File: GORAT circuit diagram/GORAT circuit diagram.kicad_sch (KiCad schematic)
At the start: 78 parts, among them J1 AudioJack2, J2 AudioJack2, J3 Conn_01x08_Socket, J4 Conn_01x08_Socket, J6 Barrel_Jack, J8 Conn_01x02_Socket, J9 Conn_01x02_Socket, Q1 J111, SW1 SW_DPDT_x2, SW8 SW_Rotary2x6, U1 OP07CP, U2 TL072ACP, U3 TL072ACP

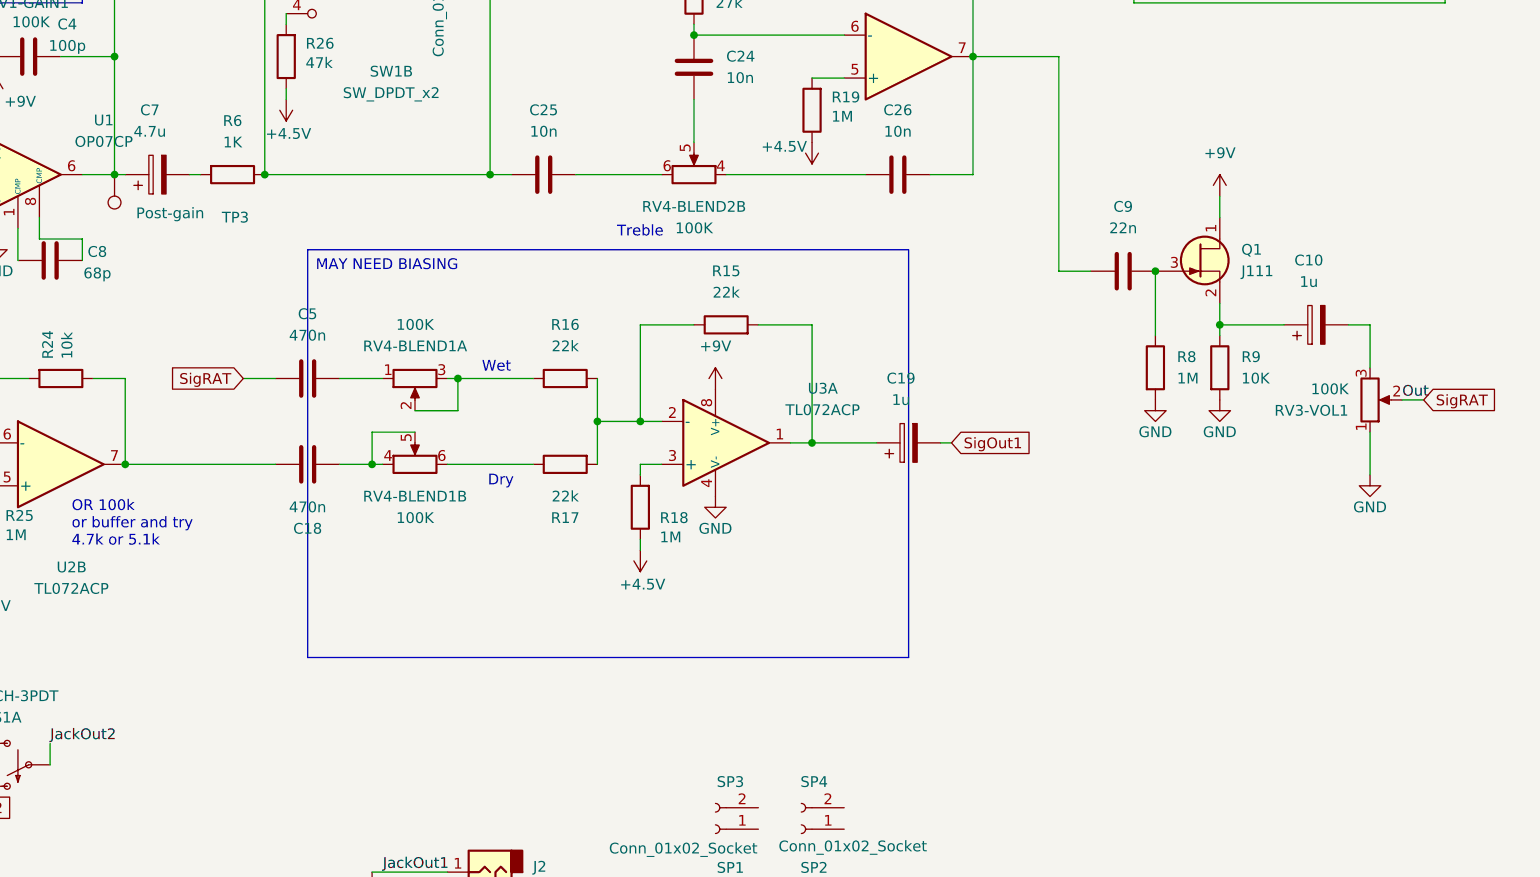
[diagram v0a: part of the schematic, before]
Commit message: potentially fixed volume mixer
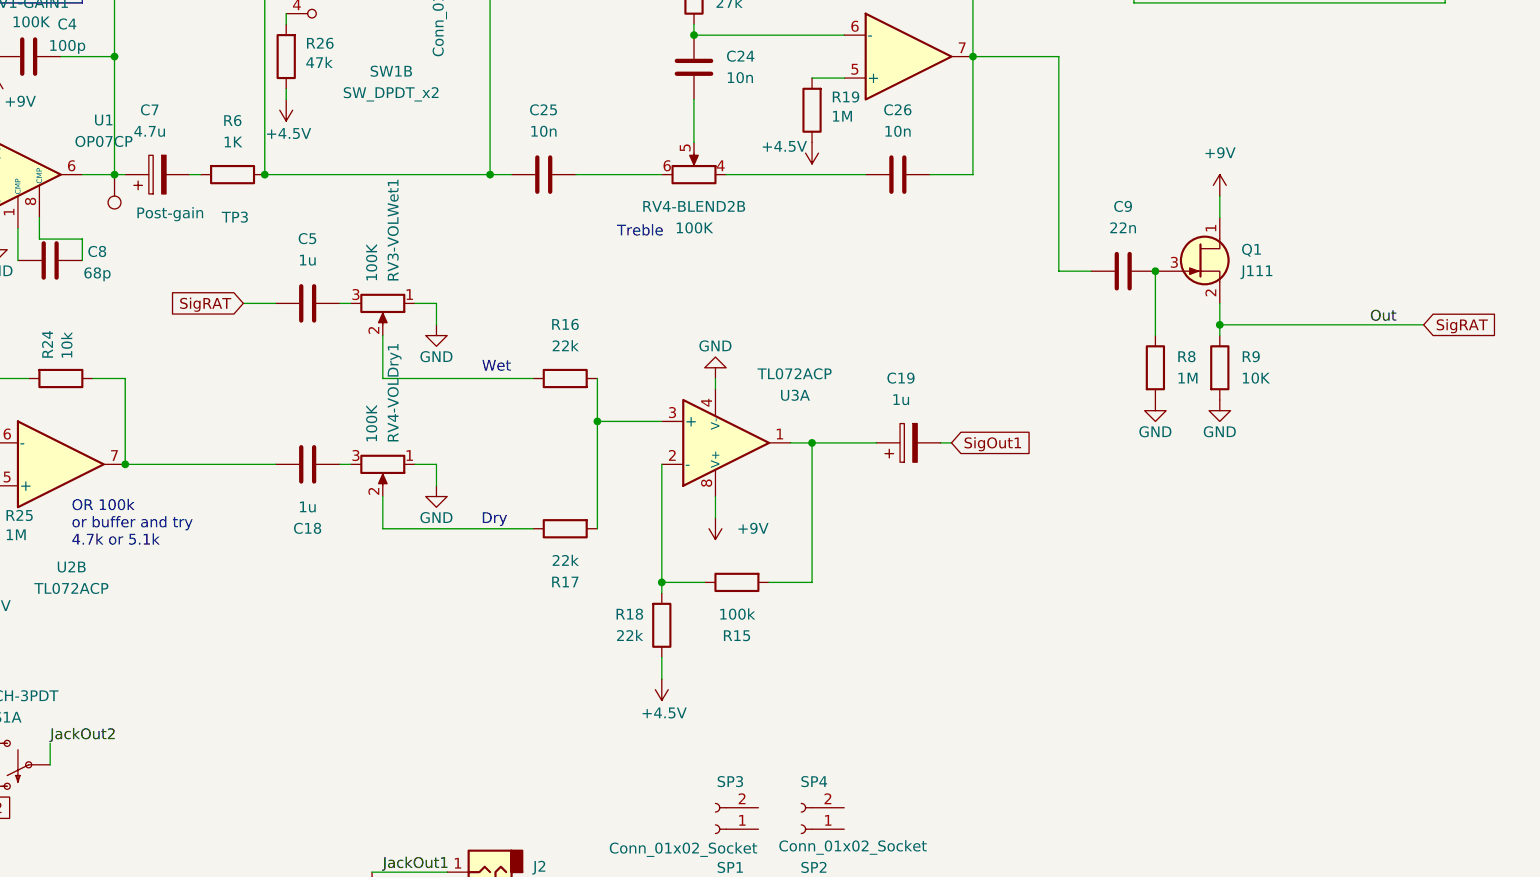
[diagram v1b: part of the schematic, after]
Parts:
- removed C10: 1u, Capacitor_THT:CP_Radial_D5.0mm_P2.50mm, symbol Device:C_Polarized
- removed RV4-BLEND1: 100K, Potentiometer_THT:Potentiometer_Alpha_RD902F-40-00D_Dual_Vertical, symbol Device:R_Potentiometer_Dual_Separate
- added RV4-VOLDry1: 100K, Daves customs:Potentiometer_Alpha_RD901F-40-00D_Single_Vertical, symbol Device:R_Potentiometer
- C18, C5: value 470n -> 1u
- R15: value 22k -> 100k
- R18: value 1M -> 22k
- renumbered RV3-VOL1 to RV3-VOLWet1
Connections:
- net GND: now also RV4-VOLDry1.1
- net SigRAT: now also Q1.2 (S), R9.1; no longer RV3-VOLWet1.2
- net at RV3-VOLWet1.3: now also C5.2
- net at R17.1: now also RV4-VOLDry1.2
- net at R16.2, R17.2: now also U3.3 (+); no longer R15.1, U3.2 (-)
- net at R16.1: now also RV3-VOLWet1.2
- net at R18.2: now also R15.1, U3.2 (-); no longer U3.3 (+)
- net at C18.2: now also RV4-VOLDry1.3
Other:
- moved on the sheet: C5, R15, R17, RV3-VOLWet1
